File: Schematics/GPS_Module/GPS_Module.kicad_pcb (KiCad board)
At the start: 4 copper layers, 69.5 x 60 mm, 68 parts, among them J1 470804001, J2 SWD_01x04_Pin, J4 Stack Male Edge Connector, J6 USB_B_Micro, Q1 AO3400A, SW1 SW_STM_RESET, SW2 SW_STM_BOOT_MODE, U1 STM32F103CBTx, U10 AMS1117-3.3, U3 W25Q128JVS, U4 LM66100DCKR, U5 LM66100DCKR, U6 LM66100DCKR, U7 ACS70331EOLC, U9 ISO1042BQDWVR, Y1 X322516MMB4SI

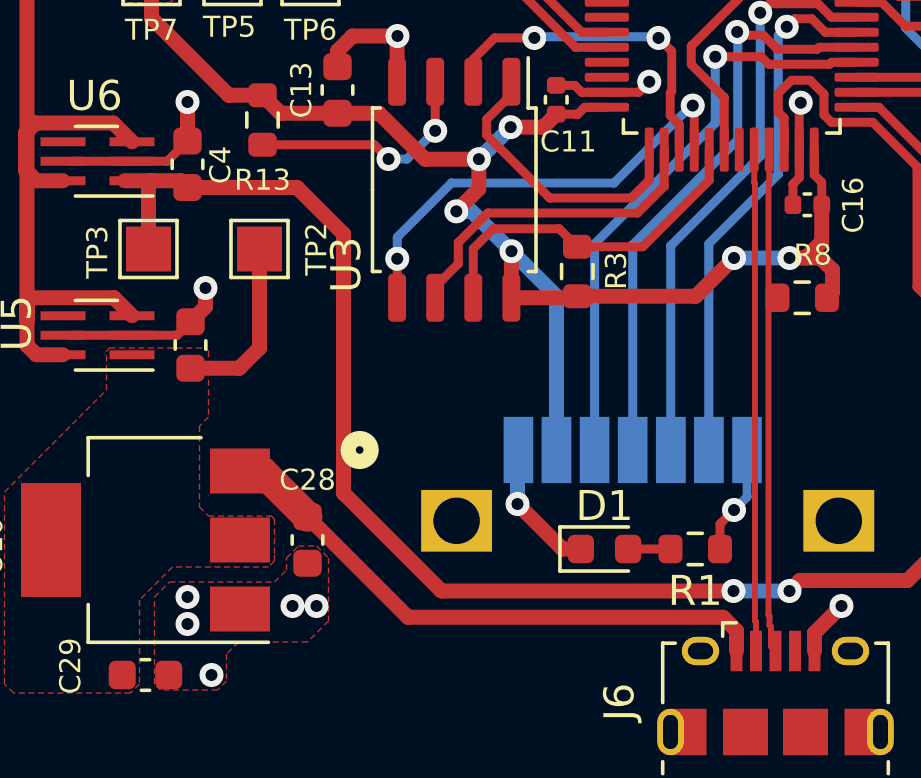
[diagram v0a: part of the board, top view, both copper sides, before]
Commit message: starting daughter board PCB layout
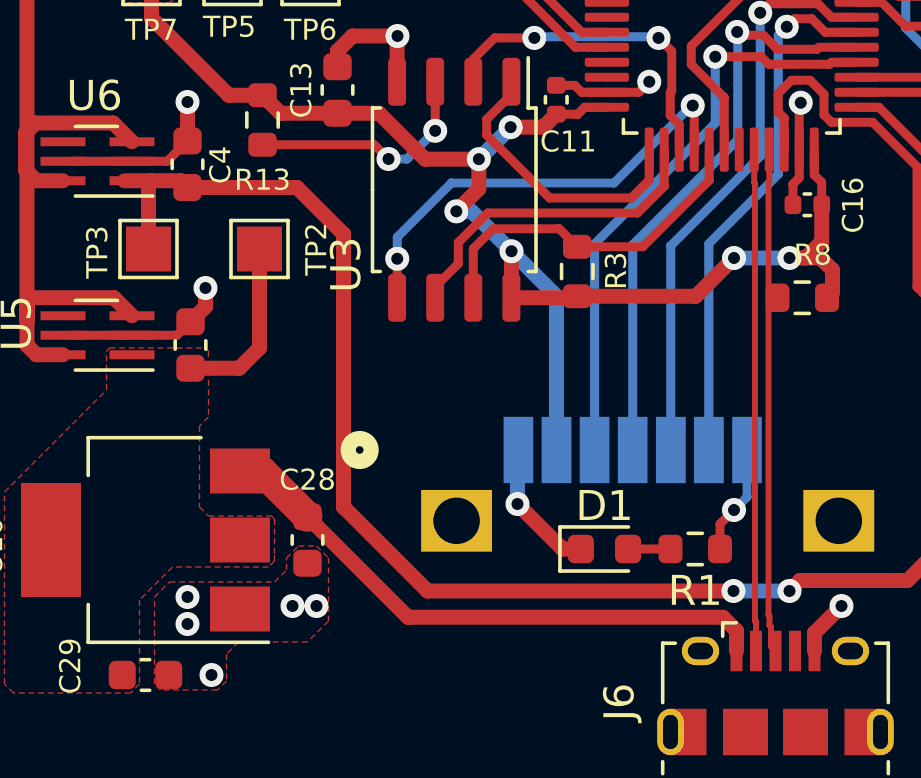
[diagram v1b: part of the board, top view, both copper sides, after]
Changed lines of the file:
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@@
   (segment (start 56.391352 50.663) (end 56.391352 49.7255) (width 0.3) (layer "F.Cu") (net 11))
   (segment (start 57.565852 73.7) (end 57.915852 73.35) (width 0.5) (layer "F.Cu") (net 12))
-  (segment (start 42.7 61.8) (end 42.7 70.436111) (width 0.5) (layer "F.Cu") (net 12))
   (segment (start 35.4 60.025) (end 36.3 60.025) (width 0.5) (layer "F.Cu") (net 12))
-  (segment (start 45.963889 73.7) (end 55.7 73.7) (width 0.5) (layer "F.Cu") (net 12))
   (segment (start 36.2 60.125) (end 36.3 60.025) (width 0.5) (layer "F.Cu") (net 12))
   (segment (start 37.275 60.025) (end 37.5 60.25) (width 0.5) (layer "F.Cu") (net 12))
+  (segment (start 42.7 70.9) (end 45.5 73.7) (width 0.5) (layer "F.Cu") (net 12))
   (segment (start 61.501472 73.35) (end 62.851472 72) (width 0.5) (layer "F.Cu") (net 12))
-  (segment (start 42.7 70.436111) (end 45.963889 73.7) (width 0.5) (layer "F.Cu") (net 12))
+  (segment (start 37.5 60.25) (end 41.15 60.25) (width 0.5) (layer "F.Cu") (net 12))
   (segment (start 36.2 62.2) (end 36.2 60.125) (width 0.5) (layer "F.Cu") (net 12))
   (segment (start 57.915852 73.35) (end 61.501472 73.35) (width 0.5) (layer "F.Cu") (net 12))
-  (segment (start 42.7 61.8) (end 41.15 60.25) (width 0.5) (layer "F.Cu") (net 12))
   (segment (start 66.985 72) (end 69.36 69.625) (width 0.5) (layer "F.Cu") (net 12))
+  (segment (start 41.15 60.25) (end 42.7 61.8) (width 0.5) (layer "F.Cu") (net 12))
+  (segment (start 42.7 61.8) (end 42.7 70.9) (width 0.5) (layer "F.Cu") (net 12))
   (segment (start 66.985 72) (end 62.851472 72) (width 0.5) (layer "F.Cu") (net 12))
-  (segment (start 41.15 60.25) (end 37.5 60.25) (width 0.5) (layer "F.Cu") (net 12))
   (segment (start 36.3 60.025) (end 37.275 60.025) (width 0.5) (layer "F.Cu") (net 12))
+  (segment (start 45.5 73.7) (end 55.7 73.7) (width 0.5) (layer "F.Cu") (net 12))
   (via (at 55.7 73.7) (size 0.8) (drill 0.4) (layers "F.Cu" "B.Cu") (net 12))
   (via (at 57.565852 73.7) (size 0.8) (drill 0.4) (layers "F.Cu" "B.Cu") (net 12))
